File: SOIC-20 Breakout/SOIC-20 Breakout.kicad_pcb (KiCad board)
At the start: 2 copper layers, 25.7 x 25.7 mm, 4 parts

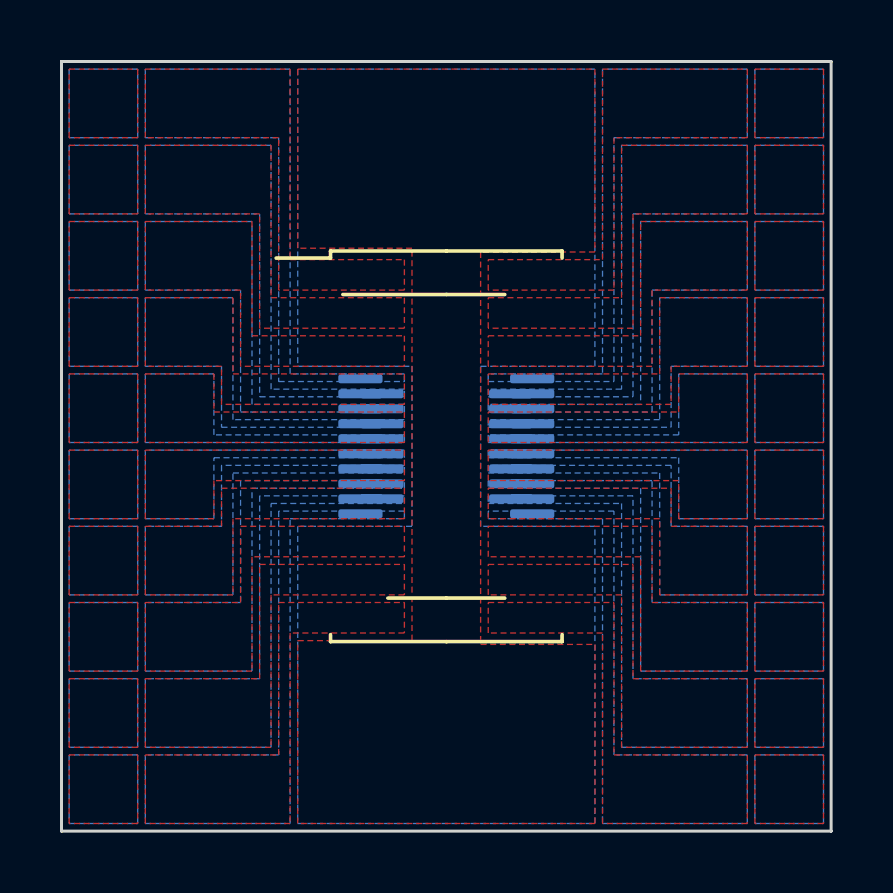
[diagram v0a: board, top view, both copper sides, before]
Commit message: Updated Files
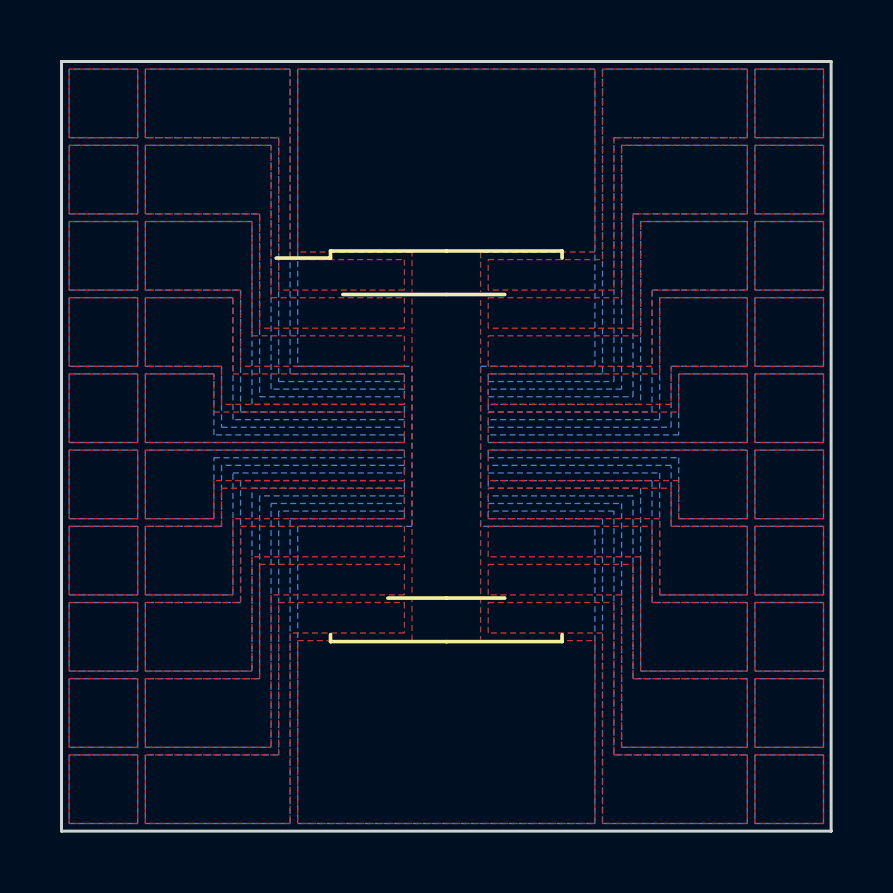
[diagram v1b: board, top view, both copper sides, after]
